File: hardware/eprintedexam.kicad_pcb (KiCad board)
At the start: 2 copper layers, 52.5 x 46.6 mm, 18 parts, among them J1 Conn_01x04, J2 Conn_01x08, SW1 SW_Push, SW2 SW_Push, U1 ESP-12F

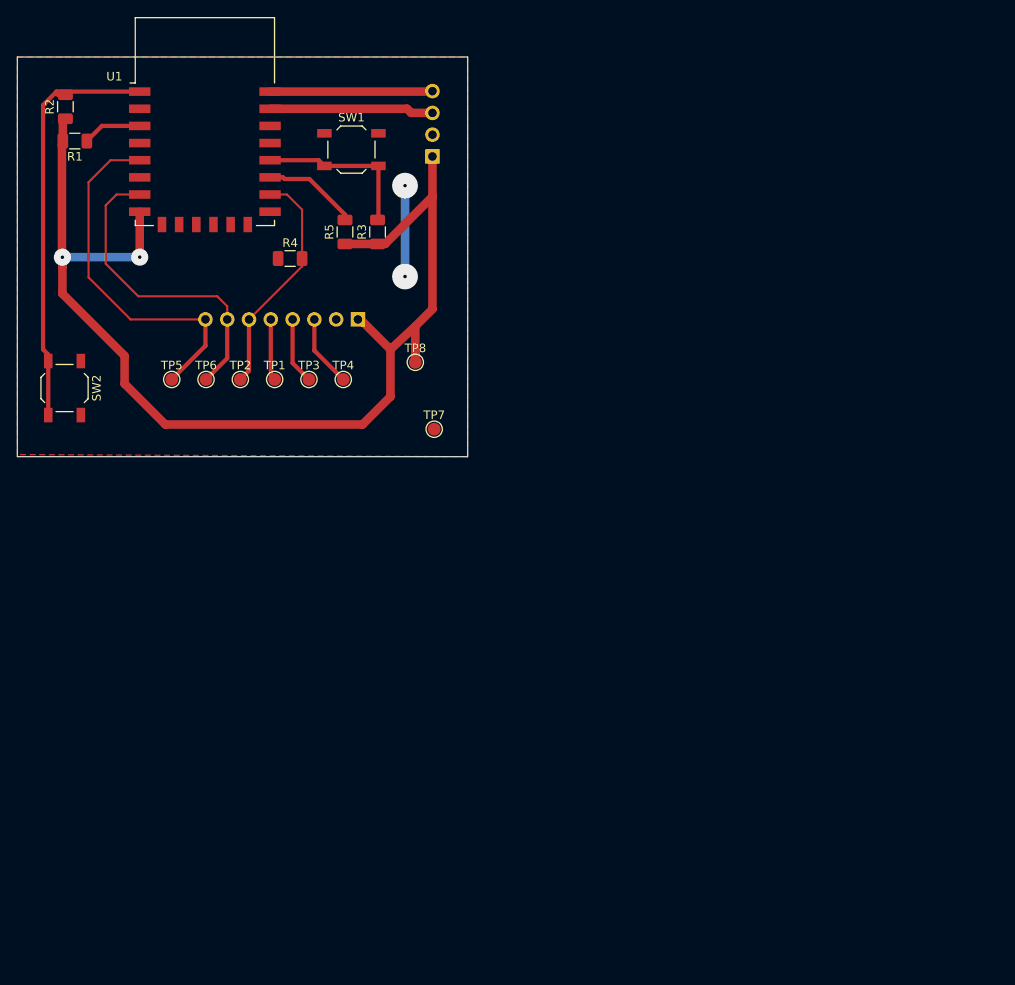
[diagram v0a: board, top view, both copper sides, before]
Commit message: mayor hardware revision
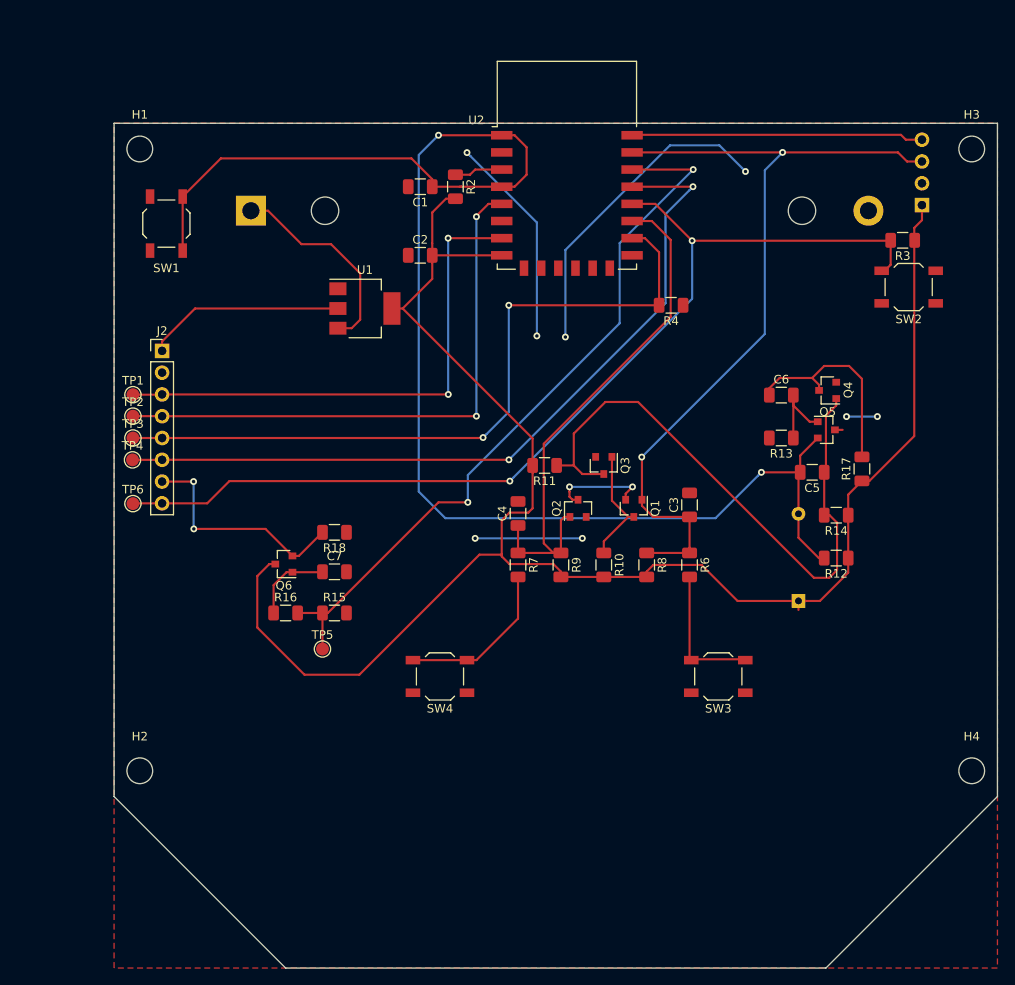
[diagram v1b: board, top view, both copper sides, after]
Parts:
- removed R1: 10k, Resistor_SMD:R_1206_3216Metric
- removed R5: R, Resistor_SMD:R_1206_3216Metric
- removed TP7, TP8: TestPoint, TestPoint:TestPoint_Pad_D1.5mm
- added BT1: Battery_Cell, Battery:BatteryHolder_MPD_BH-18650-PC2, B.Cu at (107.2, 56.3)
- added C1: 100n, Capacitor_SMD:C_1206_3216Metric, F.Cu at (127.0, 53.5)
- added C2: 100n, Capacitor_SMD:C_1206_3216Metric, F.Cu at (127.0, 61.5)
- added C3: 100n, Capacitor_SMD:C_1206_3216Metric, F.Cu at (158.4, 90.6)
- added C4: 100n, Capacitor_SMD:C_1206_3216Metric, F.Cu at (138.4, 91.6)
- added C5: 100n, Capacitor_SMD:C_1206_3216Metric, F.Cu at (172.7, 86.8)
- added C6: 10n, Capacitor_SMD:C_1206_3216Metric, F.Cu at (169.1, 77.8)
- added C7: 100n, Capacitor_SMD:C_1206_3216Metric, F.Cu at (117.0, 98.4)
- added D1: D, Diode_THT:D_DO-35_SOD27_P10.16mm_Horizontal, B.Cu at (171.1, 101.8)
- added H1: MountingHole, MountingHole:MountingHole_3mm, F.Cu at (94.3, 49.1)
- added H2: MountingHole, MountingHole:MountingHole_3mm, F.Cu at (94.3, 121.6)
- added H3: MountingHole, MountingHole:MountingHole_3mm, F.Cu at (191.3, 49.1)
- added H4: MountingHole, MountingHole:MountingHole_3mm, F.Cu at (191.3, 121.6)
- added Q1: 2N7002, Package_TO_SOT_SMD:SOT-23, F.Cu at (151.9, 91.0)
- added Q2: 2N7002, Package_TO_SOT_SMD:SOT-23, F.Cu at (145.4, 91.0)
- added Q3: 2N7002, Package_TO_SOT_SMD:SOT-23, F.Cu at (148.4, 86.0)
- added Q4: 2N7002, Package_TO_SOT_SMD:SOT-23, F.Cu at (174.3, 81.9)
- added Q5: 2N7002, Package_TO_SOT_SMD:SOT-23, F.Cu at (174.5, 77.3)
- added Q6: AO3401A, Package_TO_SOT_SMD:SOT-23, F.Cu at (111.1, 97.5)
- added R10: 33k, Resistor_SMD:R_1206_3216Metric, F.Cu at (148.4, 97.6)
- added R11: 33k, Resistor_SMD:R_1206_3216Metric, F.Cu at (141.5, 86.0)
- added R12: 10k, Resistor_SMD:R_1206_3216Metric, F.Cu at (175.5, 96.8)
- added R13: 330, Resistor_SMD:R_1206_3216Metric, F.Cu at (169.1, 82.8)
- added R14: 22k, Resistor_SMD:R_1206_3216Metric, F.Cu at (175.5, 91.8)
- added R15: 10k, Resistor_SMD:R_1206_3216Metric, F.Cu at (117.0, 103.2)
- added R16: 10k, Resistor_SMD:R_1206_3216Metric, F.Cu at (111.3, 103.2)
- added R17: 560k, Resistor_SMD:R_1206_3216Metric, F.Cu at (178.5, 86.4)
- added R18: 10k, Resistor_SMD:R_1206_3216Metric, F.Cu at (117.0, 93.8)
- added R6: 1k, Resistor_SMD:R_1206_3216Metric, F.Cu at (158.4, 97.6)
- added R7: 1k, Resistor_SMD:R_1206_3216Metric, F.Cu at (138.4, 97.6)
- added R8: 10k, Resistor_SMD:R_1206_3216Metric, F.Cu at (153.4, 97.6)
- added R9: 10k, Resistor_SMD:R_1206_3216Metric, F.Cu at (143.4, 97.6)
- added SW3: SW_Push, Button_Switch_SMD:SW_SPST_TL3342, F.Cu at (161.7, 110.6)
- added SW4: SW_Push, Button_Switch_SMD:SW_SPST_TL3342, F.Cu at (129.3, 110.6)
- added U2: ESP-12F, RF_Module:ESP-12E, F.Cu at (144.1, 51.0)
- J2: moved to F.Cu
- U1: value ESP-12F -> AP1117-33; footprint RF_Module:ESP-12E -> Package_TO_SOT_SMD:SOT-223-3_TabPin2
- moved SW2 99.1 mm to (183.9, 65.2), turned to 180 degrees
- moved R3 61.2 mm to (183.2, 59.8), turned to 180 degrees
- moved J1 57.4 mm to (185.5, 55.7)
- moved R2 46.4 mm to (131.1, 53.5), turned to 270 degrees
- moved R4 44.8 mm to (156.2, 67.3), turned to 180 degrees
- moved TP5 36.0 mm to (115.6, 107.4)
- moved U1 28.7 mm to (120.5, 67.7)
- moved TP4 26.3 mm to (93.4, 85.4)
- moved SW1 23.2 mm to (97.4, 57.8), turned to 90 degrees
- moved J2 23.1 mm to (96.9, 72.7), turned to 0 degrees
- moved TP3 21.6 mm to (93.5, 82.8)
- moved TP6 16.8 mm to (93.5, 90.5)
- moved TP1 16.6 mm to (93.5, 77.8)
- moved TP2 13.2 mm to (93.5, 80.3)
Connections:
- J1 pad 3: Net-(J1-Pad3) -> nxt
- J2 pad 3: /cs -> spi-mosi
- J2 pad 4: /dc -> spi-clk
- J2 pad 5: /rst -> spi-cs
- J2 pad 6: /busy -> spi-dc
- J2 pad 7: /mosi -> spi-nrst
- J2 pad 8: /clk -> spi-busy,flash
- R2 pad 1: VCC -> Net-(R2-Pad1)
- R2 pad 2: Net-(R2-Pad2) -> VCC
- R3 pad 2: /rst -> spi-busy,flash
- R4 pad 2: /busy -> spi-cs
- SW1 pad 2: /rst -> nrst
- SW2 pad 2: Net-(R2-Pad2) -> spi-busy,flash
- TP1 pad 1: /rst -> spi-mosi
- TP2 pad 1: /busy -> spi-clk
- TP3 pad 1: /dc -> spi-cs
- TP4 pad 1: /cs -> spi-dc
- TP5 pad 1: /clk -> spi-rst
- TP6 pad 1: /mosi -> spi-busy,flash
- U1 pad 1: Net-(R2-Pad2) -> GND
- U1 pad 2: Net-(U1-Pad2) -> VCC
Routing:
- net nrst: track 0.00 -> 172.7 mm, vias 0 -> 2
- net spi-busy,flash: track 0.00 -> 118.0 mm, vias 0 -> 2
- net nxt: track 0.00 -> 97.6 mm, vias 0 -> 2
- net spi-dc: track 0.00 -> 91.7 mm, vias 0 -> 2
- net VCC: track 134.4 -> 225.5 mm, vias 2 -> 0
- net spi-rst: track 0.00 -> 86.3 mm, vias 0 -> 2
- net spi-cs: track 0.00 -> 85.0 mm, vias 0 -> 2
- net nxt+prv: track 0.00 -> 72.3 mm
- net GND: track 10.6 -> 79.2 mm, vias 2 -> 8
- net spi-clk: track 0.00 -> 66.9 mm, vias 0 -> 2
- net prv: track 0.00 -> 62.6 mm
- net spi-mosi: track 0.00 -> 61.3 mm, vias 0 -> 2
- net Net-(R2-Pad2): track 49.6 -> 0.00 mm
- net /clk: track 42.6 -> 0.00 mm
- net /mosi: track 37.1 -> 0.00 mm
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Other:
- board size 52.5 x 46.6 mm -> 103 x 98.5 mm
